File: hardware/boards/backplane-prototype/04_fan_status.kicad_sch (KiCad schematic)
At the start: 14 parts, among them J11 12V 3-WIRE FAN, J12 DS18B20 EXT SUPPLY, J9 12V 3-WIRE FAN, Q1 AO3407A, Q2 2N7002, Q3 AO3407A, Q4 2N7002

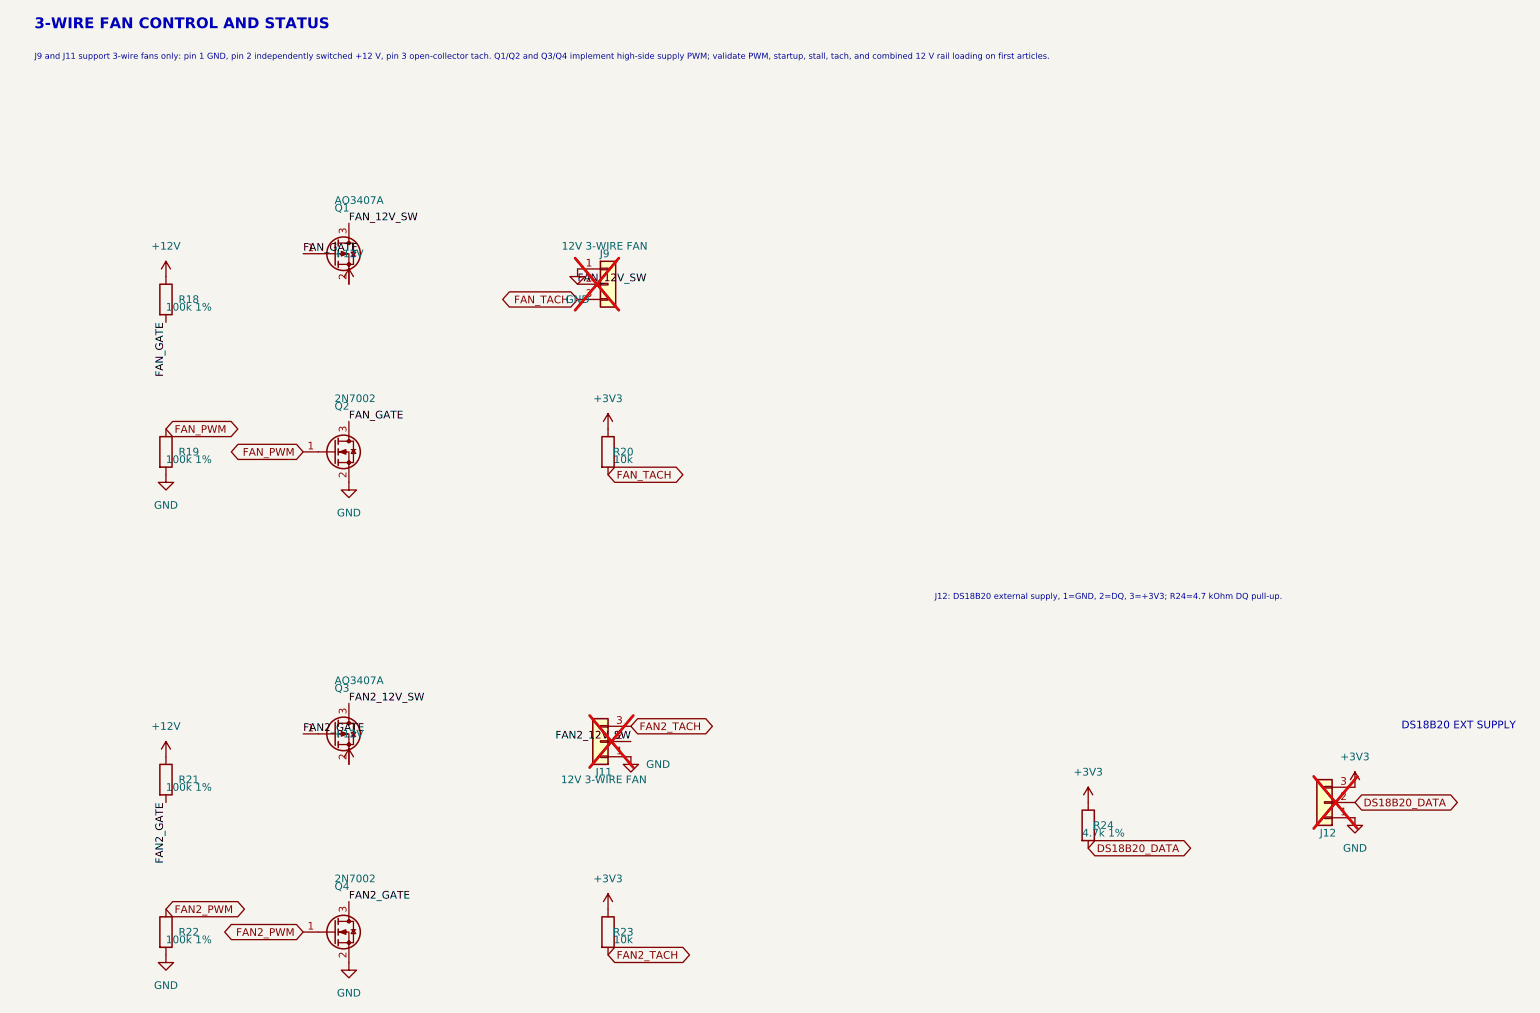
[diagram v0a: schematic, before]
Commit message: checkpoint: save fan schematic layout
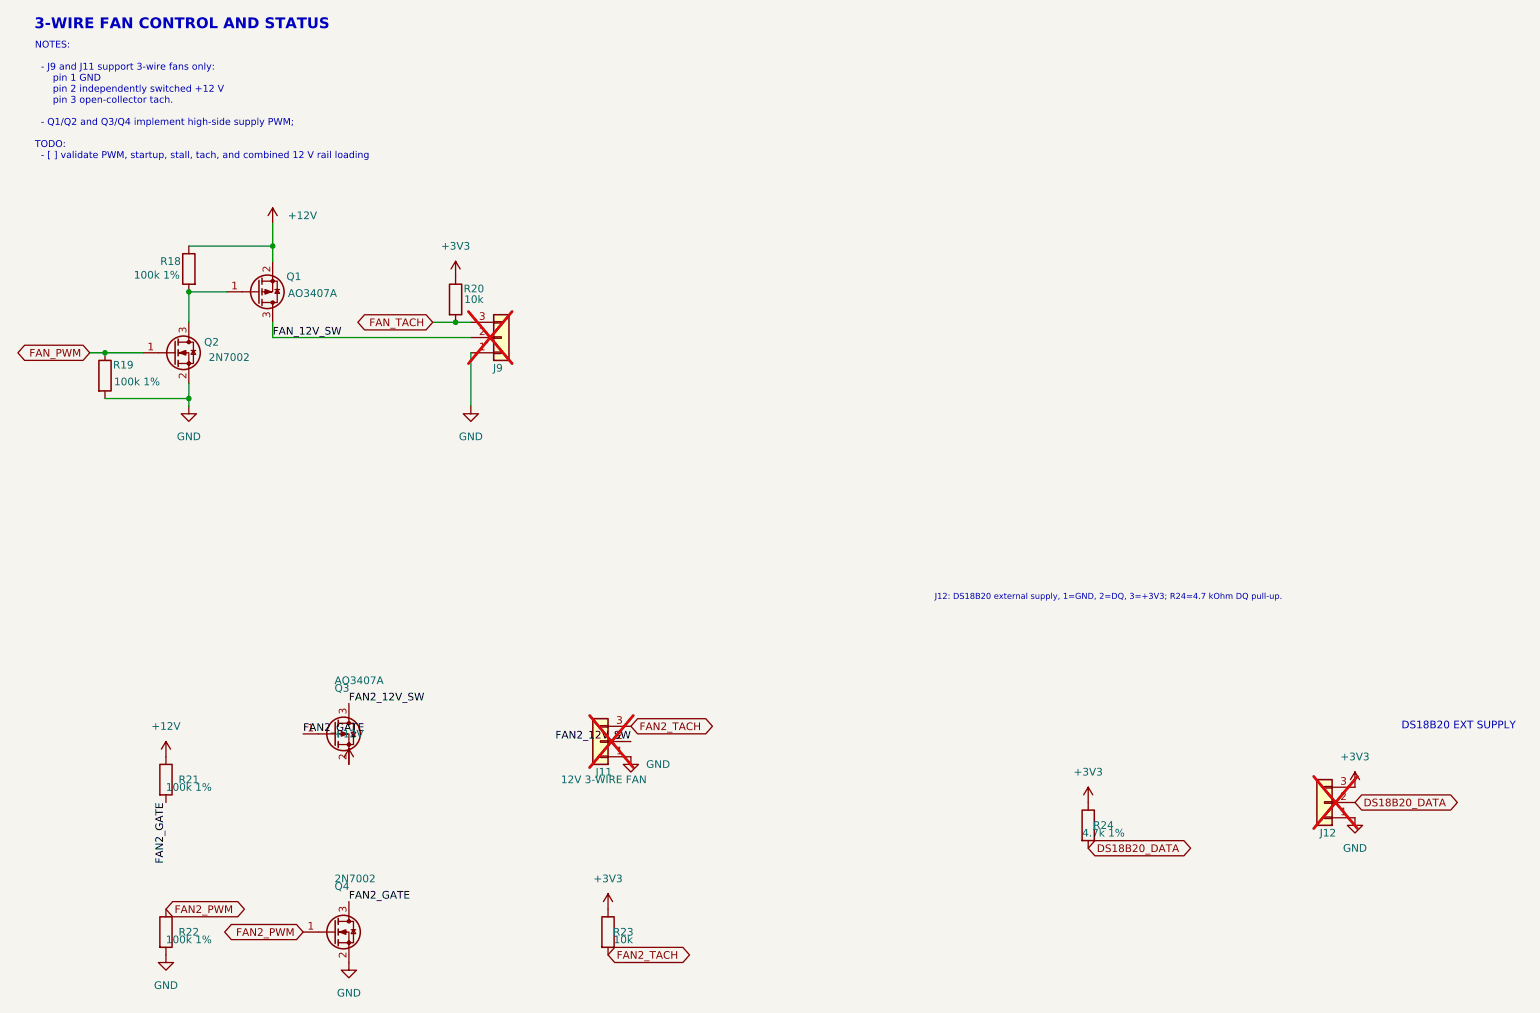
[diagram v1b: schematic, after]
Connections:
- net FAN_GATE: no longer names the net of Q1.1 (G), Q2.3 (D), R18.2
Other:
- note added: "NOTES: - J9 and J11 support 3-wire fans only: pin 1 GND pin 2 independently switched +12 V pin 3 open-collector tach. - Q1/Q2 and Q3/Q4 implement high-side supply PWM; TODO: - [ ] validate PWM, startup, stall, tach, and combined 12 V rail loading"
- note removed: "J9 and J11 support 3-wire fans only: pin 1 GND, pin 2 independently switched +12 V, pin 3 open-collector tach. Q1/Q2 and Q3/Q4 implement high-side supply PWM; validate PWM, startup, stall, tach, and combined 12 V rail loading on first articles."
- moved on the sheet: J9, Q1, Q2, R18, R19, R20
